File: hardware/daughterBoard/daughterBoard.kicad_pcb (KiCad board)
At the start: 4 copper layers, 24 x 36 mm, 44 parts, among them J1 Conn_02x05_Top_Bottom, J2 Conn_02x02_Odd_Even, J3 Conn_02x02_Odd_Even, J4 Conn_02x05_Top_Bottom, U1 DRV2605LDGSR, U2 TCA9544APWR, U3 VL53L1CXV0FY1, U4 DRV2605LDGSR, U5 IS31FL3193-DLS2-TR

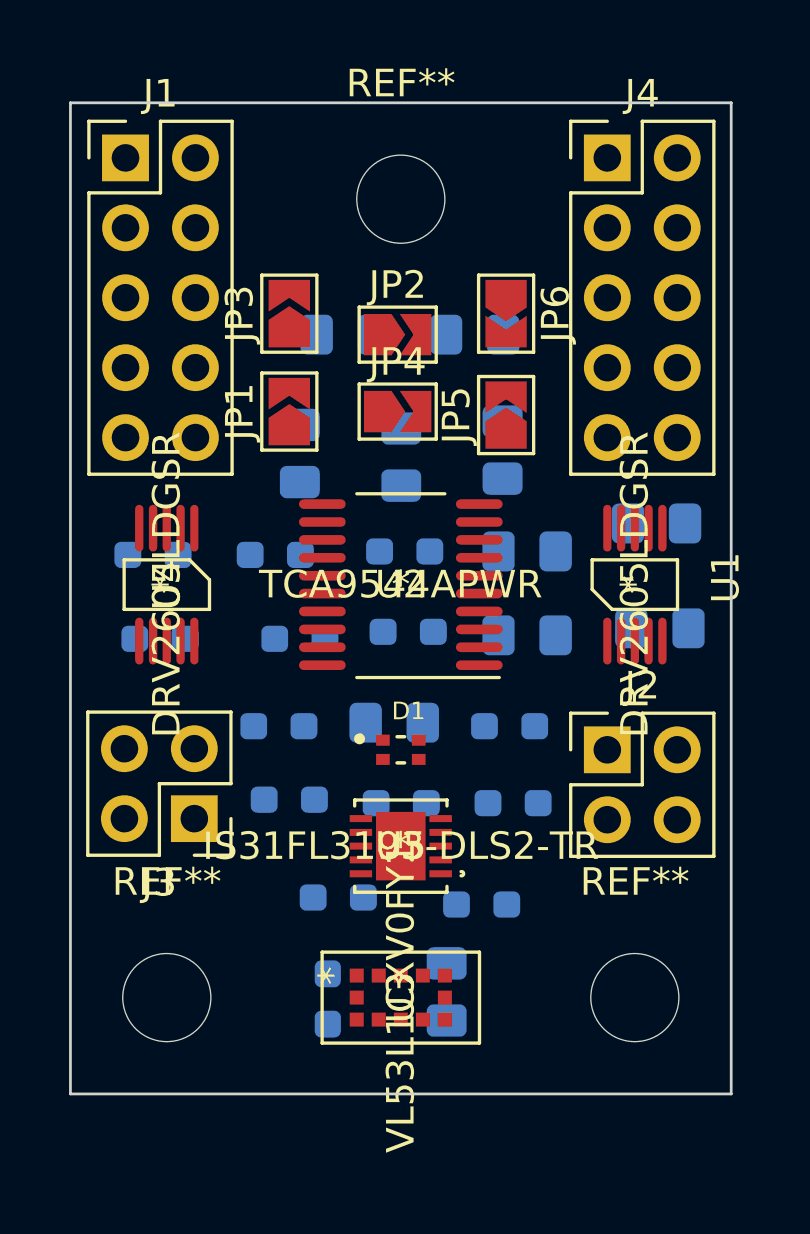
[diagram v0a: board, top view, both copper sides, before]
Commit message: v1 finished
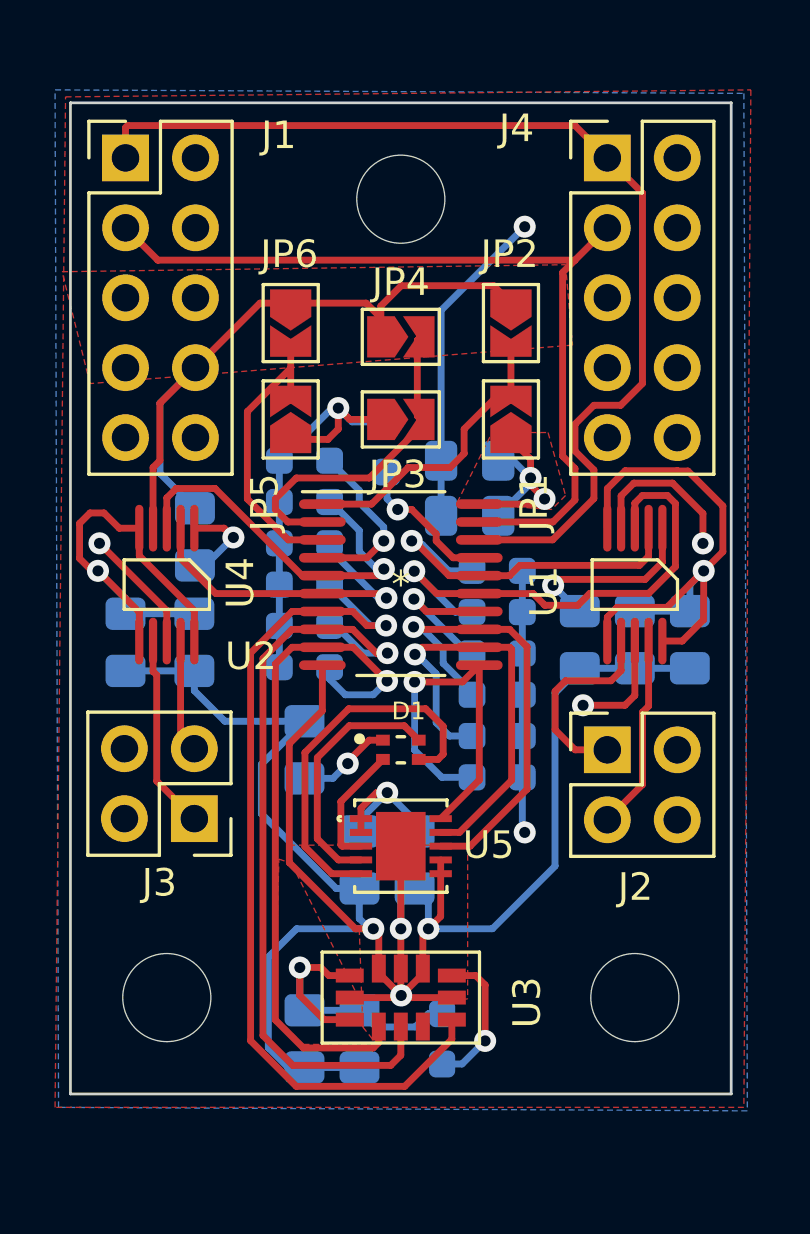
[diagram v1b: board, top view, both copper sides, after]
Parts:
- added C12: .1u, Capacitor_SMD:C_0805_2012Metric_Pad1.18x1.45mm_HandSolder, B.Cu at (114.5, 63.0)
- added C13: 1u, Capacitor_SMD:C_0805_2012Metric_Pad1.18x1.45mm_HandSolder, B.Cu at (114.5, 65.0)
- J1, J4: value Conn_02x05_Top_Bottom -> Conn_02x05_Odd_Even
- moved C8 22.7 mm to (108.5, 84.0), turned to -90 degrees
- moved C4 19.4 mm to (102.0, 69.6), turned to -90 degrees
- moved C10 19.1 mm to (110.5, 77.5), turned to 90 degrees
- moved R1 18.6 mm to (113.5, 84.0), turned to -90 degrees
- moved C11 15.3 mm to (112.5, 77.5), turned to 90 degrees
- moved R12 13.3 mm to (108.5, 64.5)
- moved C5 13.2 mm to (104.5, 69.6)
- moved R7 12.6 mm to (115.5, 71.5), turned to 0 degrees
- moved C1 12.4 mm to (122.5, 69.5)
- moved R14 12.3 mm to (115.5, 70.0)
- moved C6 12.1 mm to (104.5, 65.8), turned to 90 degrees
- moved C3 11.7 mm to (118.5, 69.5), turned to -90 degrees
- moved C9 11.6 mm to (110.5, 84.0), turned to -90 degrees
- moved R3 11.4 mm to (108.5, 67.5)
- moved R4 10.9 mm to (111.5, 62.5), turned to -90 degrees
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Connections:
- net Net-(U2-Pad14) renamed /INT3
- C7 pad 1: unconnected-(C7-Pad1) -> +3V3
- J1 pad 2: /SDM -> unconnected-(J1-Pad2)
- J1 pad 3: +3V3 -> /SDM
- J1 pad 4: GND -> unconnected-(J1-Pad4)
- J1 pad 5: unconnected-(J1-Pad5) -> +3V3
- J1 pad 6: unconnected-(J1-Pad6) -> +3V3
- J1 pad 7: unconnected-(J1-Pad7) -> GND
- J1 pad 8: unconnected-(J1-Pad8) -> GND
- J4 pad 2: /SDM -> unconnected-(J4-Pad2)
- J4 pad 3: +3V3 -> /SDM
- J4 pad 4: GND -> unconnected-(J4-Pad4)
- J4 pad 5: unconnected-(J4-Pad5) -> +3V3
- J4 pad 6: unconnected-(J4-Pad6) -> +3V3
- J4 pad 7: unconnected-(J4-Pad7) -> GND
- J4 pad 8: unconnected-(J4-Pad8) -> GND
- R13 pad 2: Net-(U2-Pad11) -> /INT2
- R2 pad 1: /INT0 -> +3V3
- R2 pad 2: +3V3 -> /INT0
- U1 pad 2: /SC2 -> /SC3
- U1 pad 3: /SD2 -> /SD3
- U2 pad 11: Net-(U2-Pad11) -> /INT2
- U3 pad 10: /SC0 -> /SC1
- U3 pad 7: /INT0 -> /INT1
- U3 pad 9: /SD0 -> /SD1
- U4 pad 2: /SC3 -> /SC0
- U4 pad 3: /SD3 -> /SD0
- U5 pad 10: /INT1 -> /INT2
- U5 pad 8: /SC1 -> /SC2
- U5 pad 9: /SD1 -> /SD2
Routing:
- net GND: track 0.00 -> 132.9 mm, vias 0 -> 8
- net +3V3: track 0.00 -> 94.8 mm, vias 0 -> 9
- net /SCM: track 0.00 -> 38.7 mm
- net /INT1: track 0.00 -> 31.9 mm, vias 0 -> 1
- net /SDM: track 0.00 -> 31.4 mm
- net /SD1: track 0.00 -> 28.2 mm, vias 0 -> 1
- net /SC1: track 0.00 -> 25.5 mm, vias 0 -> 1
- net /SD3: track 0.00 -> 18.2 mm, vias 0 -> 1
- net /SC2: track 0.00 -> 17.1 mm, vias 0 -> 1
- net /SD2: track 0.00 -> 16.1 mm, vias 0 -> 1
- net /SD0: track 0.00 -> 14.2 mm, vias 0 -> 1
- net Net-(D1-Pad3): track 0.00 -> 13.8 mm
- net /INT2: track 0.00 -> 13.7 mm, vias 0 -> 1
- net /SC3: track 0.00 -> 13.1 mm, vias 0 -> 1
- net /SC0: track 0.00 -> 12.2 mm, vias 0 -> 1
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- added copper zone on B.Cu, net (none)
- added copper zone on F.Cu, net (none)
- added copper zone on F.Cu, net +3V3
- added copper zone on In2.Cu, net +3V3
- added copper zone on F.Cu, net GND
- added copper zone on In1.Cu, net GND
